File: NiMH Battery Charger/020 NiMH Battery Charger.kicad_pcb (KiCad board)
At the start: 2 copper layers, 100 x 72.8 mm, 103 parts, among them J1 USB_C_Receptacle_PowerOnly_6P, U1 AMS1117-3.3, U2 ESP32-WROOM-32D, U3 AMS1117-3.3, U4 D168K

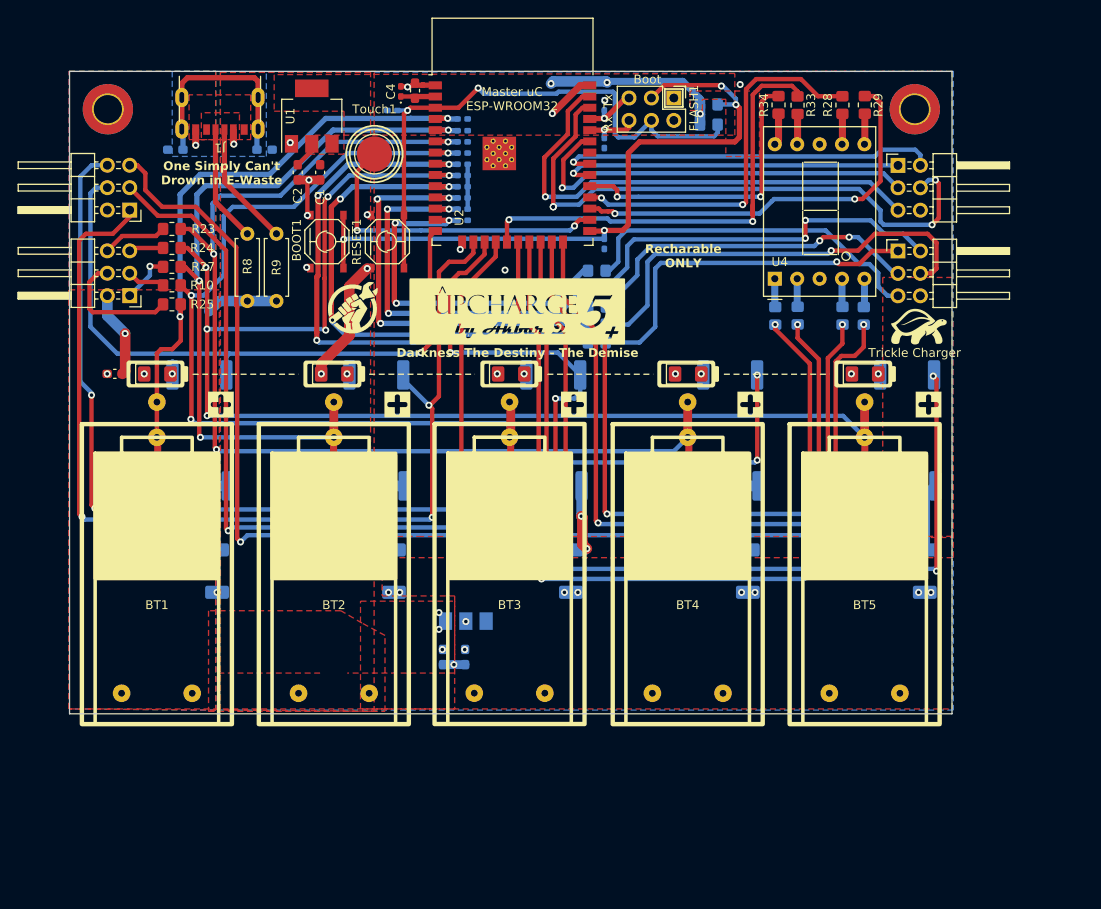
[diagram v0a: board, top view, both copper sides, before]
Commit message: Re-Print Main PCB File
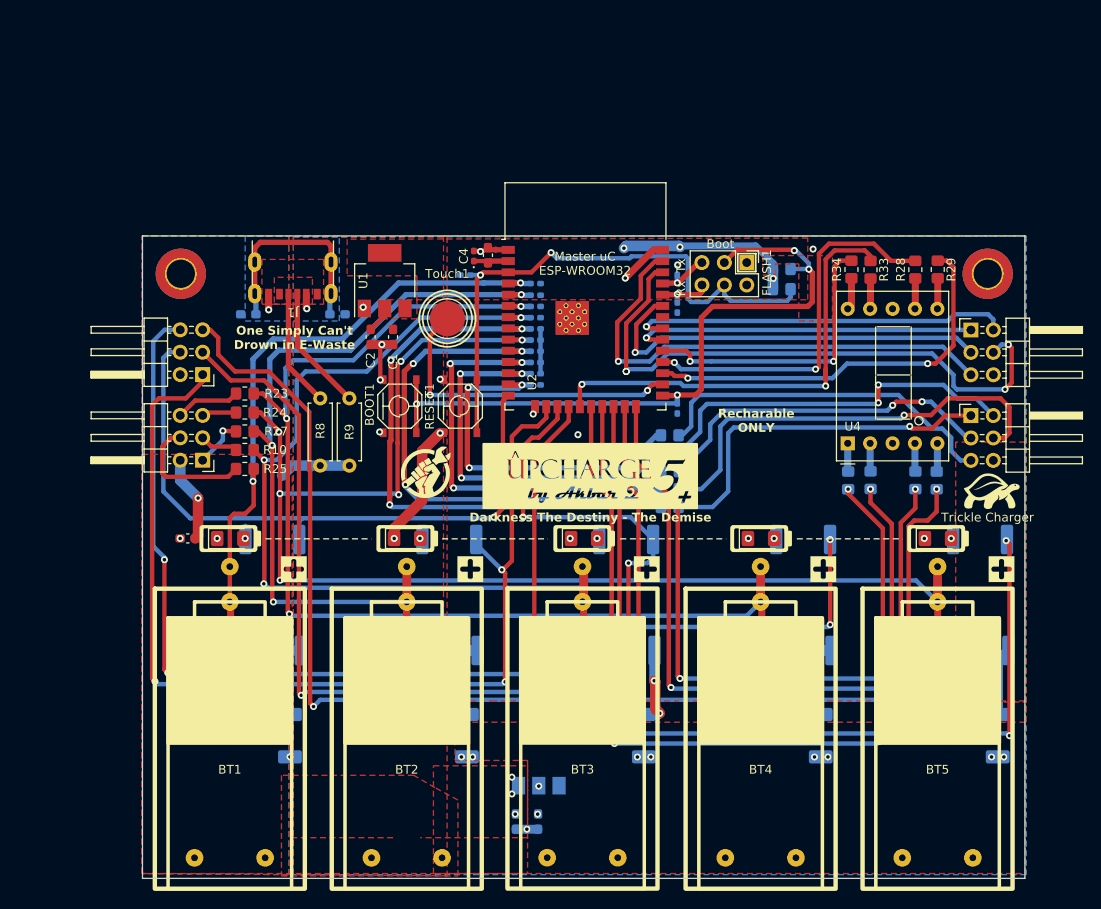
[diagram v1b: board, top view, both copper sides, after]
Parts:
- moved BT1 20.4 mm to (34.2, 106.2)
- moved BT2 20.4 mm to (54.3, 106.2)
- moved BT3 20.4 mm to (74.2, 106.2)
- moved BT4 20.4 mm to (94.4, 106.2)
- moved BT5 20.4 mm to (114.4, 106.2)
- moved D21 20.4 mm to (61.1, 95.4)
- moved D22 20.4 mm to (41.0, 95.4)
- moved D23 20.4 mm to (81.1, 95.4)
- moved D24 20.4 mm to (101.2, 95.4)
- moved D25 20.4 mm to (121.2, 95.4)
- moved G*** 20.4 mm to (41.5, 76.5)
- moved G*** 20.4 mm to (56.3, 65.5)
- moved G*** 20.4 mm to (121.7, 76.5)
- moved G*** 20.4 mm to (56.0, 63.1)
- moved G*** 20.4 mm to (74.1, 99.7)
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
